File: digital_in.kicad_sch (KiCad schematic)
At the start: 16 parts, among them U1401 CDSOT236-T05, U1402 AM26LV32E, U1403 CDSOT236-T05

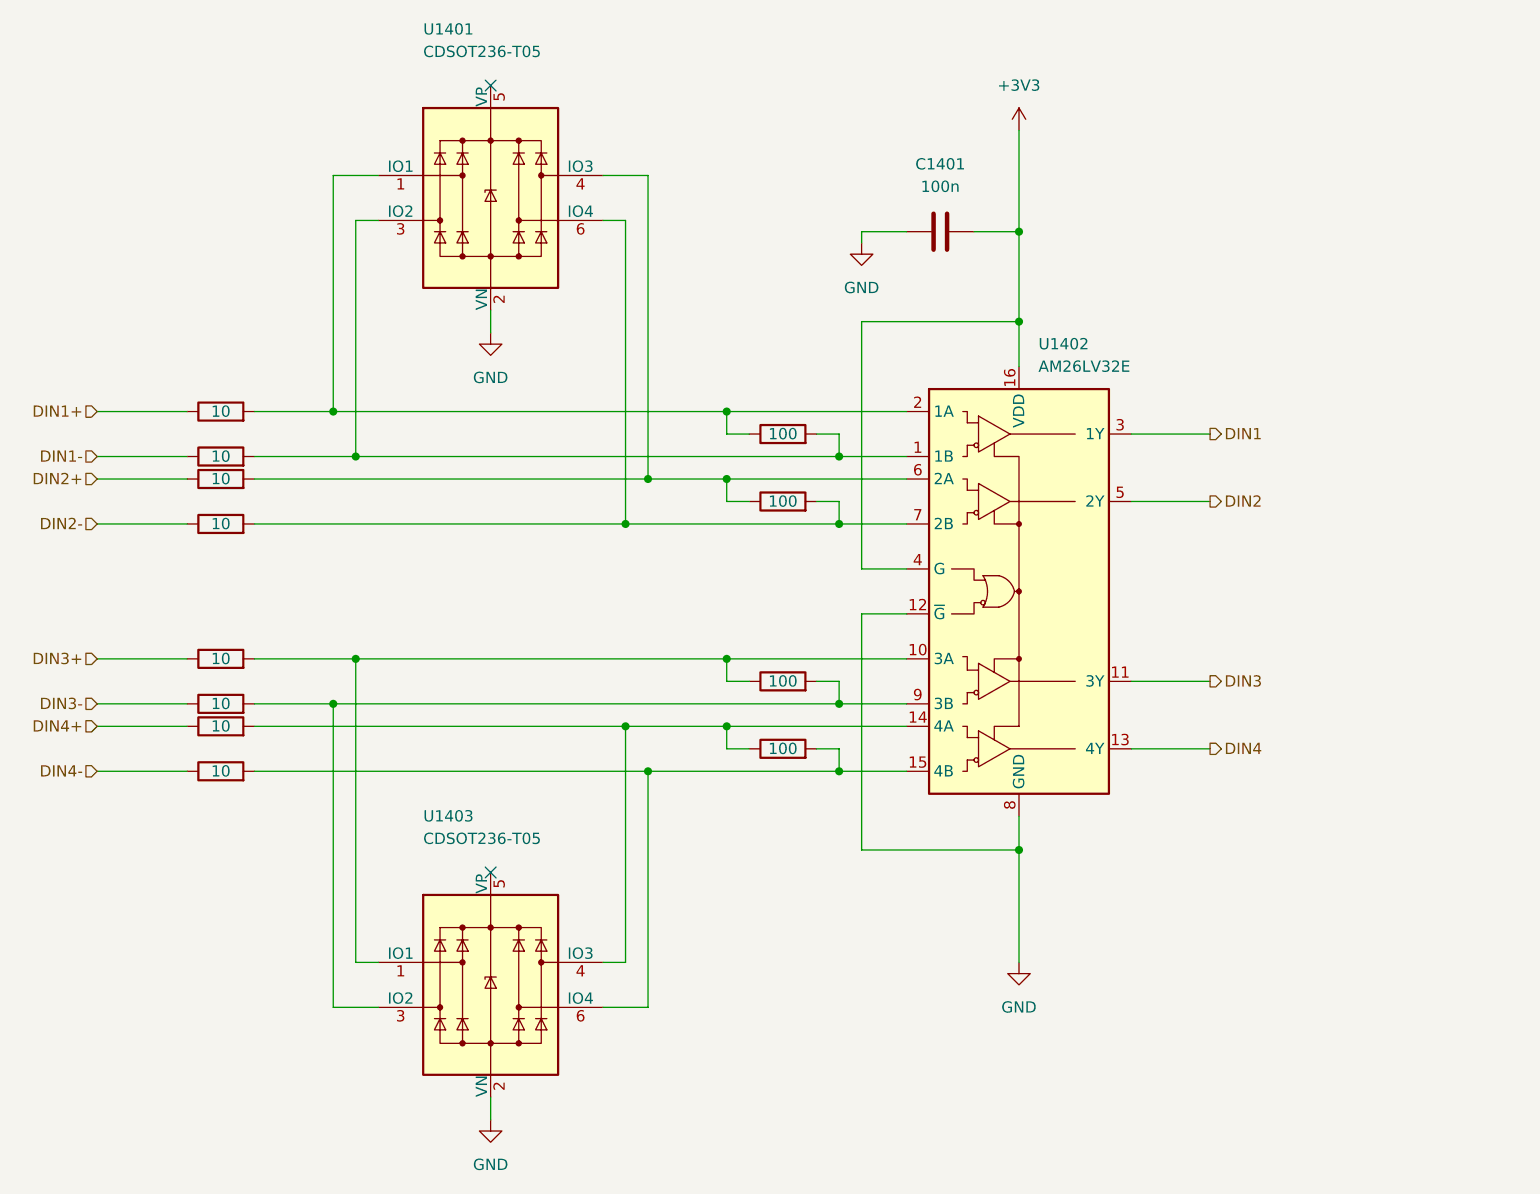
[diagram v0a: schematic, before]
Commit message: Fixed ERC errors and warnings
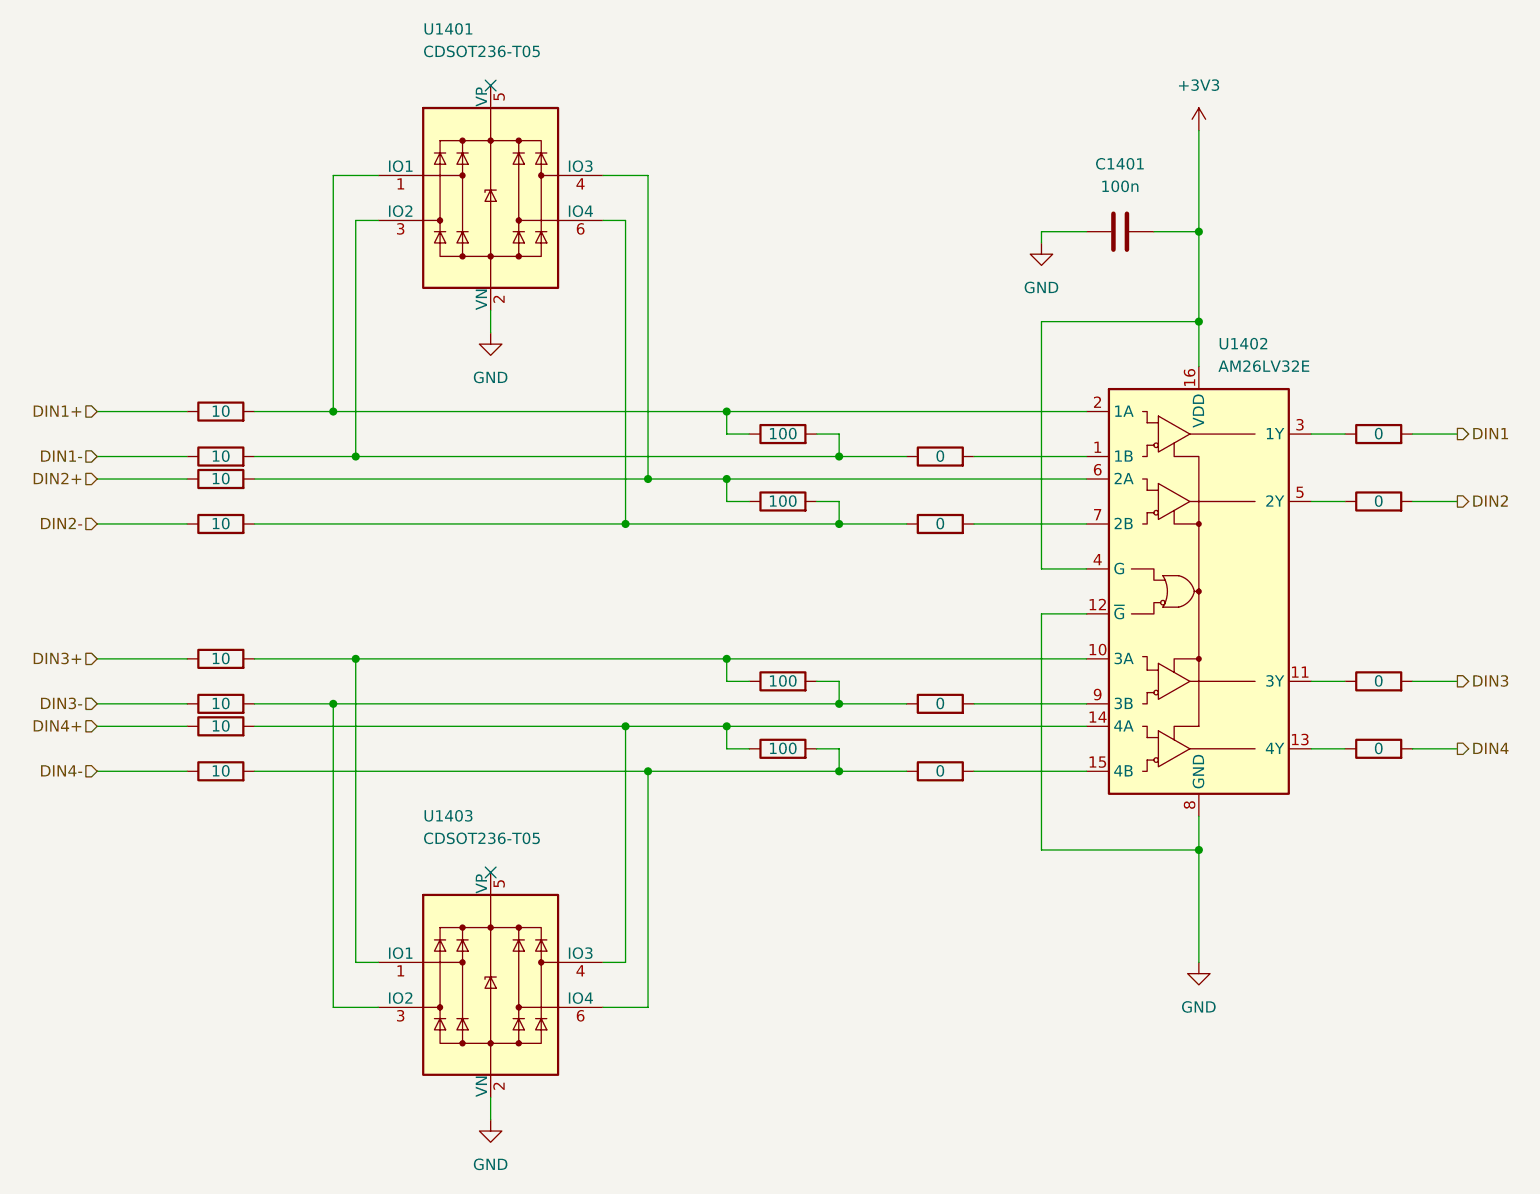
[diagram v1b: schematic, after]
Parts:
- added R1103, R1105, R1108, R1110, R1113, R1115, R1118, R1120: 0, Resistor_SMD:R_0603_1608Metric_Pad0.98x0.95mm_HandSolder, symbol Device:R
- renumbered R1403 to R1404, R1404 to R1406, R1405 to R1407, R1406 to R1409, R1407 to R1411, R1408 to R1412, R1409 to R1414, R1410 to R1416, R1411 to R1417, R1412 to R1419
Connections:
- net DIN1: now also R1103.2; no longer U1402.3 (1Y)
- net DIN2: now also R1108.2; no longer U1402.5 (2Y)
- net DIN3: now also R1113.2; no longer U1402.11 (3Y)
- net DIN4: now also R1118.2; no longer U1402.13 (4Y)
- net at R1417.2, R1419.2, U1403.6 (IO4): now also R1120.1; no longer U1402.15 (4B)
- net at R1412.2, R1414.2, U1403.3 (IO2): now also R1115.1; no longer U1402.9 (3B)
- net at R1407.2, R1409.2, U1401.6 (IO4): now also R1110.1; no longer U1402.7 (2B)
- net at R1402.2, R1404.2, U1401.3 (IO2): now also R1105.1; no longer U1402.1 (1B)
- new net: R1118.1, U1402.13 (4Y)
- new net: R1105.2, U1402.1 (1B)
- new net: R1113.1, U1402.11 (3Y)
- new net: R1120.2, U1402.15 (4B)
- new net: R1103.1, U1402.3 (1Y)
- new net: R1108.1, U1402.5 (2Y)
- new net: R1110.2, U1402.7 (2B)
- new net: R1115.2, U1402.9 (3B)
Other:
- moved on the sheet: C1401, U1402
